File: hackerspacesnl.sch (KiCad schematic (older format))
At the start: 54 parts, among them J1 Screw_Terminal_01x02, J2 Conn_01x04_Male, Q1 Q_NMOS_GSD, Q2 Q_NMOS_GSD, Q3 Q_NMOS_GSD, Q4 Q_NMOS_GSD, Q5 Q_NMOS_GSD, Q6 Q_NMOS_GSD, SW1 SW_Push, SW2 SW_Push, U1 AMS1117-3.3, U2 ESP32-wroom-32

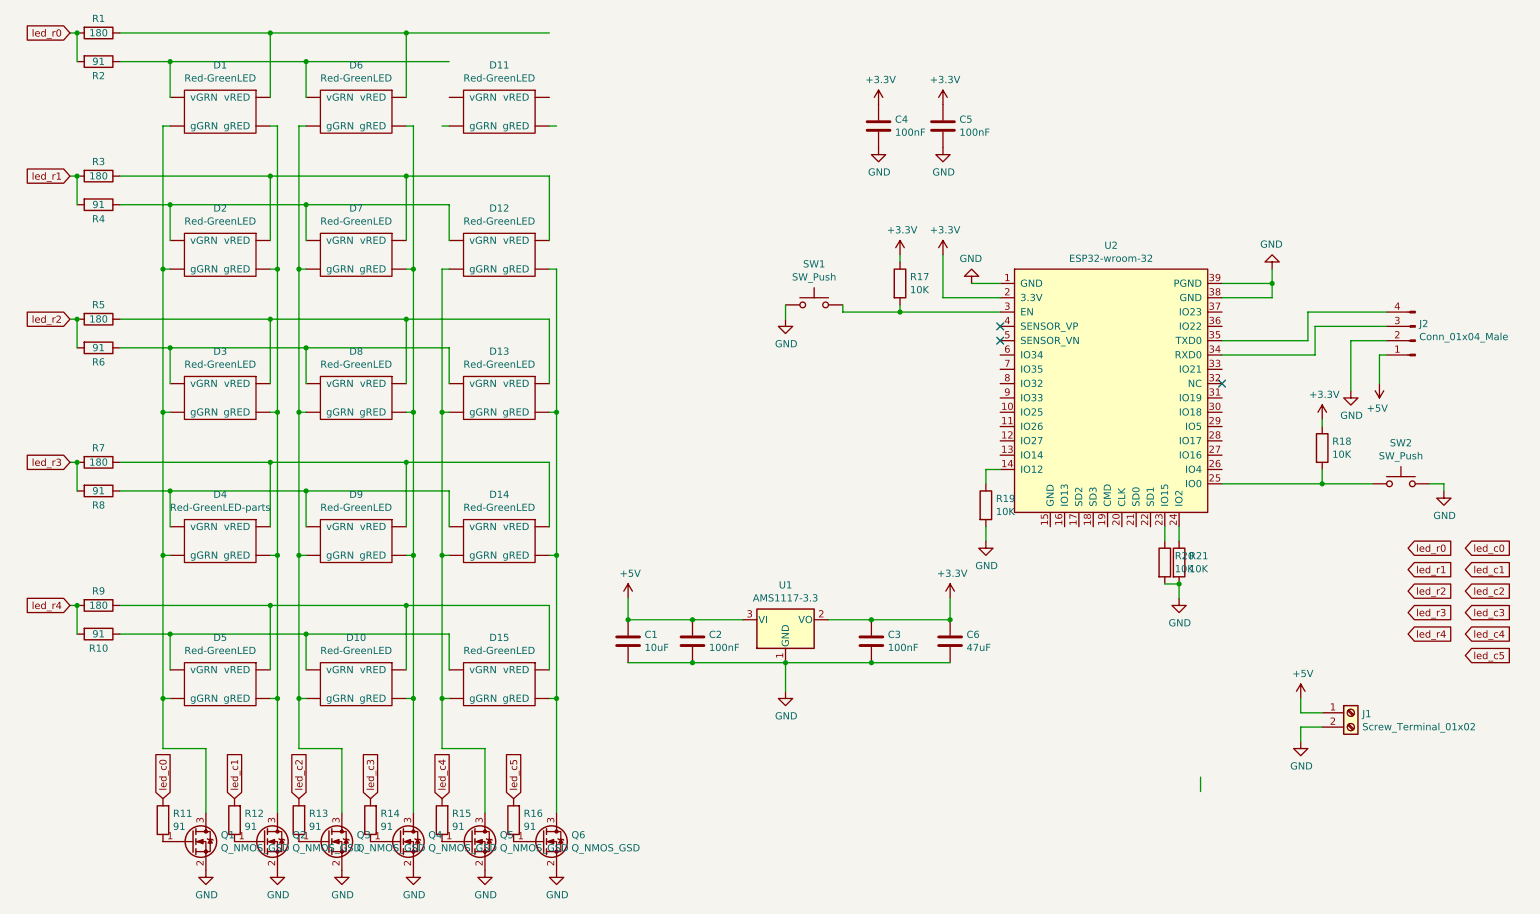
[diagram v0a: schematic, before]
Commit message: layout almost done
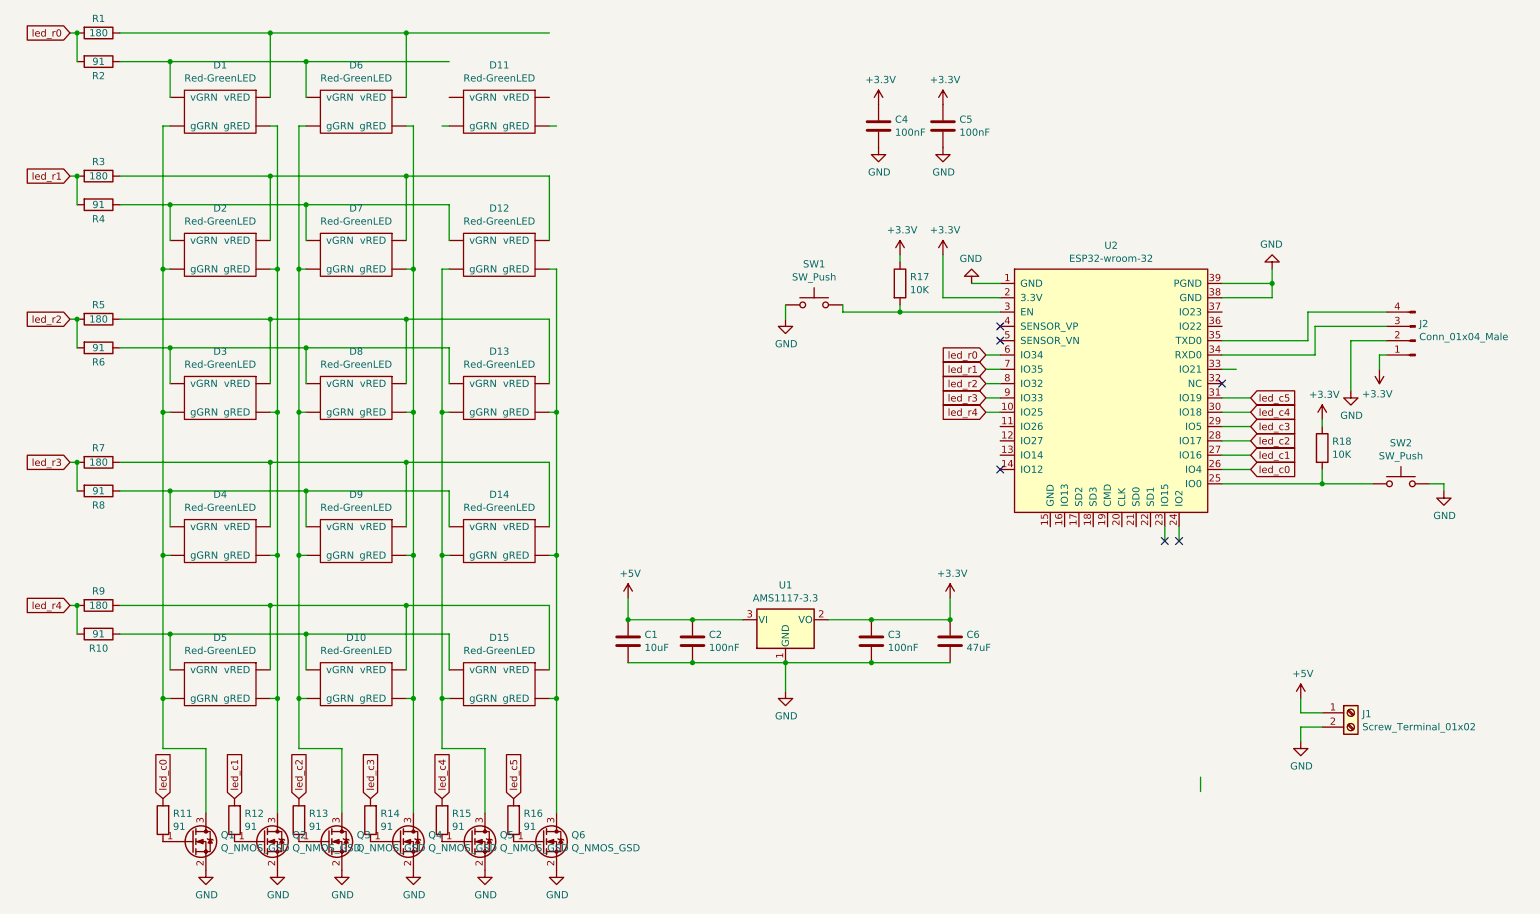
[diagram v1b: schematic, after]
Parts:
- removed R19, R20, R21: 10K, Resistor_SMD:R_0603_1608Metric, symbol Device:R
- C1: LCSC (none) -> C19702
- C2, C3, C4, C5: LCSC (none) -> C14663
- C6: LCSC (none) -> C108053
- D1, D10, D11, D12, D13, D14, D15, D2, D3, D5, D6, D7, D8, D9: LCSC (none) -> C391863
- D4: value Red-GreenLED-parts -> Red-GreenLED; LCSC (none) -> C391863
- Q1, Q2, Q3, Q4, Q5, Q6: LCSC (none) -> C181087
- R1, R3, R5, R7, R9: LCSC (none) -> C22828
- R10, R11, R12, R13, R14, R15, R16, R2, R4, R6, R8: LCSC (none) -> C25199
- R17, R18: LCSC (none) -> C25804
- U1: LCSC (none) -> C351784
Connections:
- wire segments 184 -> 191
- no-connect marks 3 -> 6

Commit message: versie zoals besteld
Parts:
- C6: LCSC C108053 -> C16780
- U1: LCSC C351784 -> C6186
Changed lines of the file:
@@
 F 2 "Package_TO_SOT_SMD:SOT-223-3_TabPin2" H 5850 5100 50  0001 C CNN
 F 3 "http://www.advanced-monolithic.com/pdf/ds1117.pdf" H 5950 4650 50  0001 C CNN
-F 4 "C351784" H 5850 4900 50  0001 C CNN "LCSC"
+F 4 "C6186" H 5850 4900 50  0001 C CNN "LCSC"
 	1    5850 4900
 	1    0    0    -1
@@
 F 2 "Capacitor_SMD:C_0805_2012Metric" H 7038 4900 50  0001 C CNN
 F 3 "~" H 7000 5050 50  0001 C CNN
-F 4 "C108053" H 7000 5050 50  0001 C CNN "LCSC"
+F 4 "C16780" H 7000 5050 50  0001 C CNN "LCSC"
 	1    7000 5050
 	1    0    0    -1

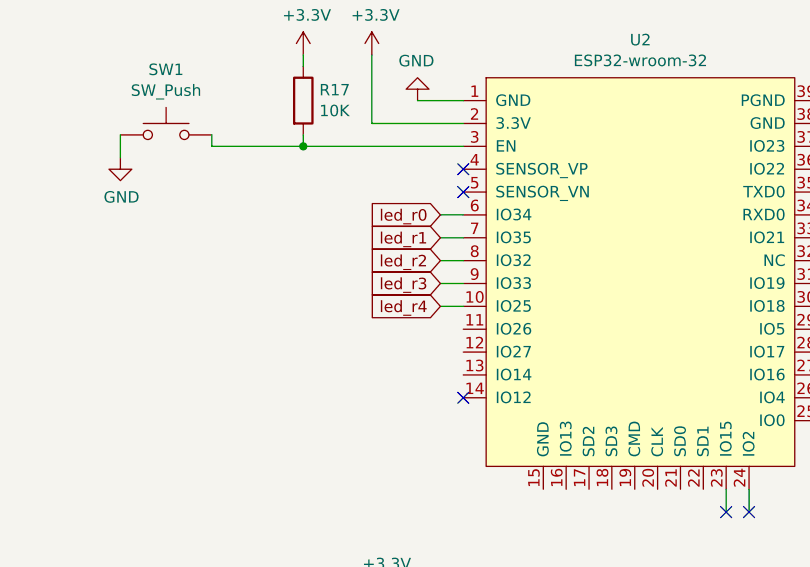
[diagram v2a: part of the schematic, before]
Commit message: nieuwe rev
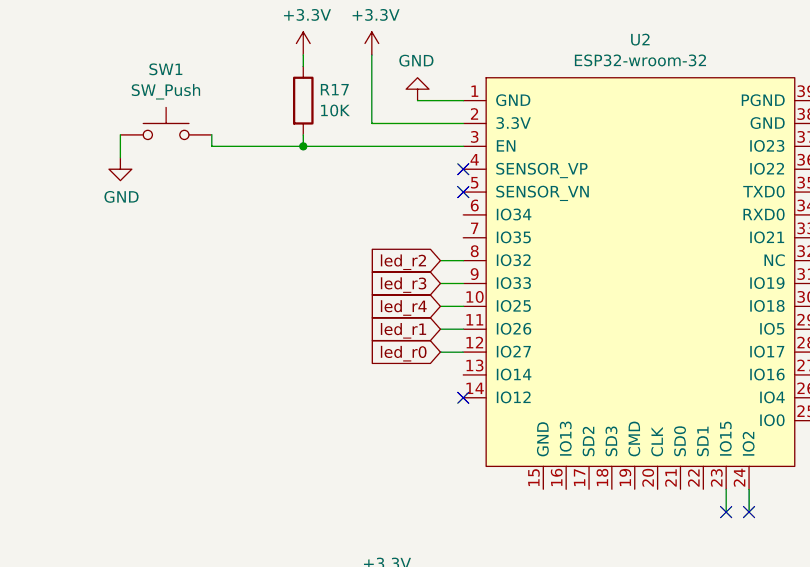
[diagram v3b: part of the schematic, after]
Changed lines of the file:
@@
 	1    0    0    -1
 $EndComp
-Text GLabel 7250 3150 0    50   Input ~ 0
+Text GLabel 7250 3550 0    50   Input ~ 0
 led_r1
 Text GLabel 7250 3250 0    50   Input ~ 0
@@
 Wire Wire Line
 	9600 3500 9600 3550
-Text GLabel 7250 3050 0    50   Input ~ 0
+Text GLabel 7250 3650 0    50   Input ~ 0
 led_r0
 Wire Wire Line
@@
 	9000 3150 8900 3150
 Wire Wire Line
-	7350 3050 7250 3050
-Wire Wire Line
-	7250 3150 7350 3150
-Wire Wire Line
 	7350 3250 7250 3250
 Wire Wire Line
@@
 Wire Wire Line
 	8900 3850 9100 3850
+Wire Wire Line
+	7250 3550 7350 3550
+Wire Wire Line
+	7350 3650 7250 3650
 $EndSCHEMATC
